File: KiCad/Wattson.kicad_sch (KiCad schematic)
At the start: 16 parts, among them J1 DC, J2 USB A, J3 Banana/Spade, J4 Banana/Spade, J5 USB A, J6 Spade/Banana/Alligator, J7 Spade/Banana/Alligator, M1 24V, SW1 Power On, U1 Power Monitor VIN, U2 Power Monitor VADJ, U3 LM317 Regulator (VADJ 5-22VDC)

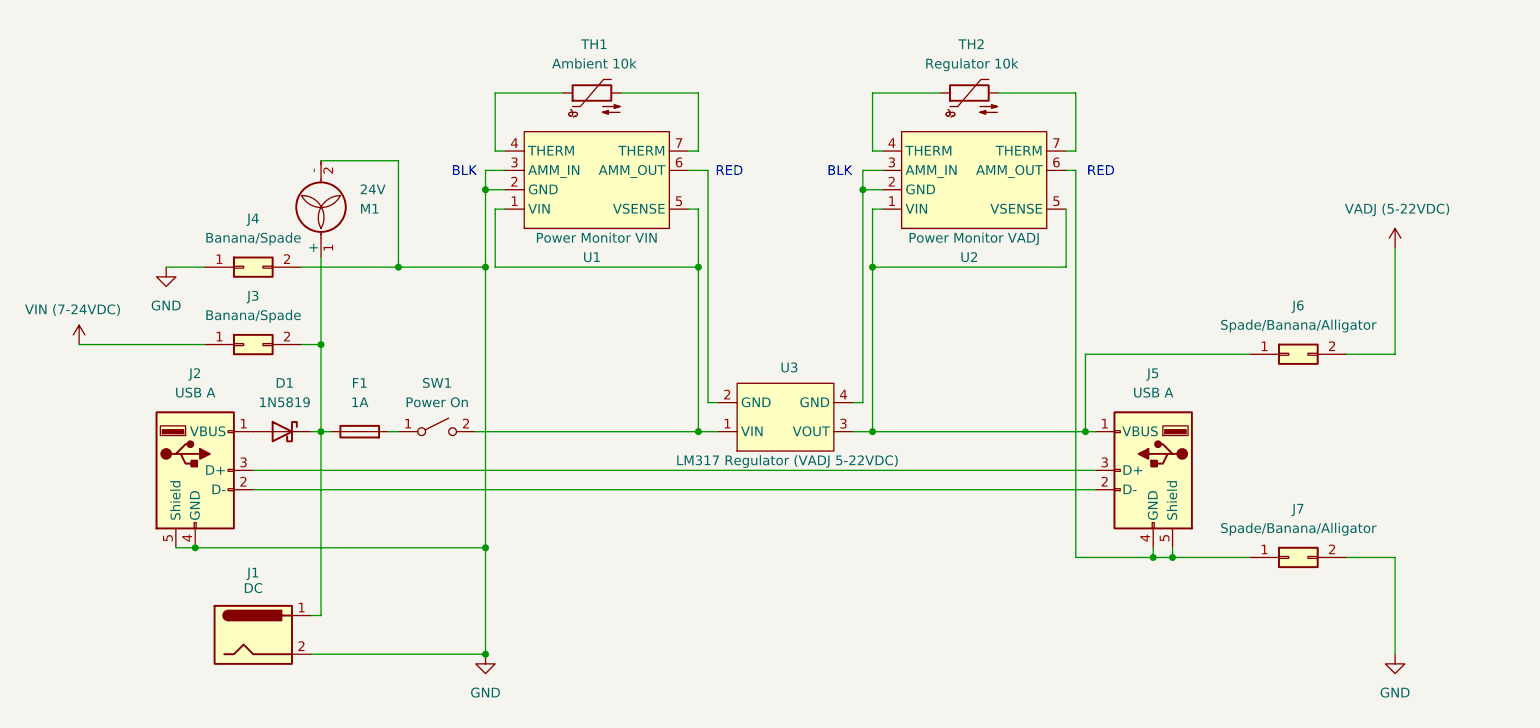
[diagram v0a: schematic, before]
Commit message: Update Wattson
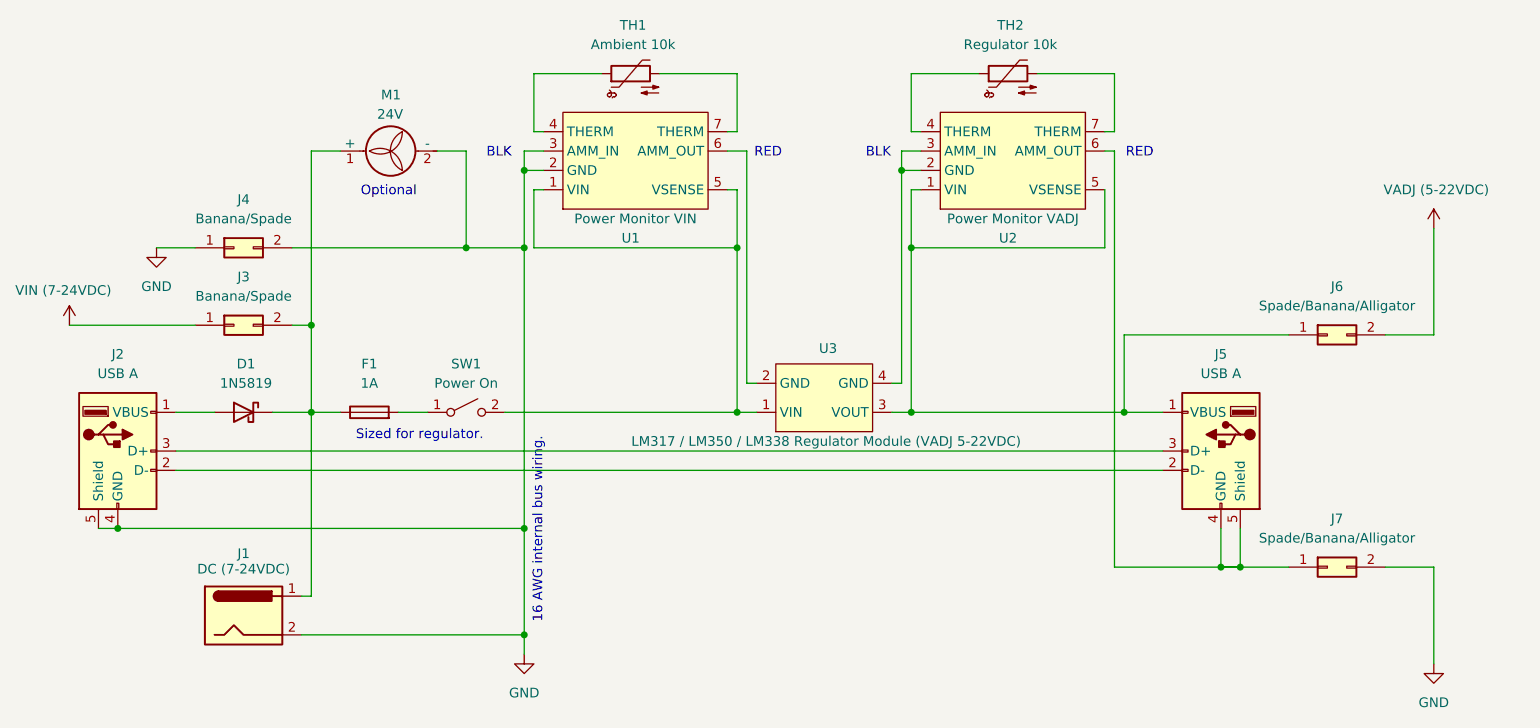
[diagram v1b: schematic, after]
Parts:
- J1: value DC -> DC (7-24VDC)
- U3: value LM317 Regulator (VADJ 5-22VDC) -> LM317 / LM350 / LM338 Regulator Module (VADJ 5-22VDC)
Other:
- note added: "16 AWG internal bus wiring."
- note added: "Optional"
- note added: "Sized for regulator."
- moved on the sheet: D1, F1, J1, J2, J3, J4, J5, J6, J7, M1, SW1, TH1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
